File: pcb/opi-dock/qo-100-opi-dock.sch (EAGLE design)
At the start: 115 parts, among them CON1 6P-SH-SIDE, CON10 4P-SH-SIDE, CON11 3P-SH-SIDE, CON12 3P-SH-SIDE, CON13 4P-SH-SIDE, CON19 2P-PH-TOP, CON2 6P-SH-SIDE, CON20 2EDG-2P-5MM, CON3 3P-SH-SIDE, CON4 4P-SH-SIDE, CON5 4P-SH-SIDE, CON6 4P-SH-SIDE, CON7 4P-SH-SIDE, CON8 4P-SH-SIDE, CON9 4P-SH-SIDE, Q1 AO3400, U1 ORANGEPIZERO, U11 DS2484, U12 LTC4313-1, U13 MCP1525, U14 MIC23155, U15 LT8640S, U16 MCP3221-A0, U17 LTC4313-1, U2 MCP1703-500, U3 MCP23008, U4 LTC4313-2, U5 ADUM1250, U6 MCP1703-500, U7 MCP23008, U8 LTC4313-2, U9 ADUM1250

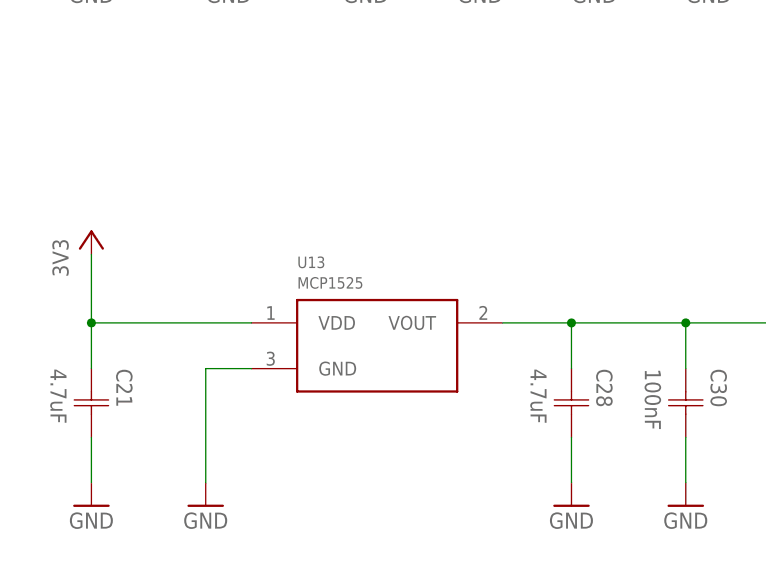
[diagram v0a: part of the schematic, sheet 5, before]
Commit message: Work on PCBs
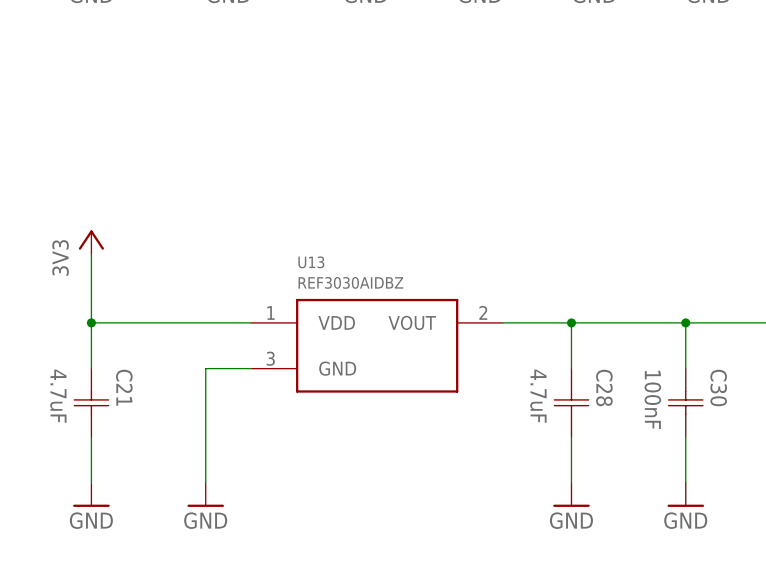
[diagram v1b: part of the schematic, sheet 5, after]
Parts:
- U13: value MCP1525 -> REF3030AIDBZ; device Microchip:MCP1525 -> Texas Instruments:REF3030AIDBZ
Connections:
- net 2V5_ADC_CLEAN renamed 3V0_ADC_CLEAN
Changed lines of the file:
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@@
 <part name="U11" library="Maxim Integrated" deviceset="DS2484" device=""/>
 <part name="U16" library="Microchip" deviceset="MCP3221-A*" device="" technology="0"/>
-<part name="U13" library="Microchip" deviceset="MCP1525" device=""/>
+<part name="U13" library="Texas Instruments" deviceset="REF30*AIDBZ" device="" technology="30"/>
 <part name="3V64" library="Supply Symbol" deviceset="3V3" device=""/>
 <part name="GND45" library="Supply Symbol" deviceset="GND" device=""/>
@@
 </segment>
 </net>
-<net name="2V5_ADC_CLEAN" class="0">
+<net name="3V0_ADC_CLEAN" class="0">
 <segment>
 <pinref part="U16" gate="G$1" pin="VDD"/>
